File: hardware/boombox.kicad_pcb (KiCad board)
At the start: 2 copper layers, 13 parts, among them J1 Micro_SD_Card_Det1, J5 AudioJack4, U7 MCP7940MT-I/SN, U9 MCP73811T-420I-OT

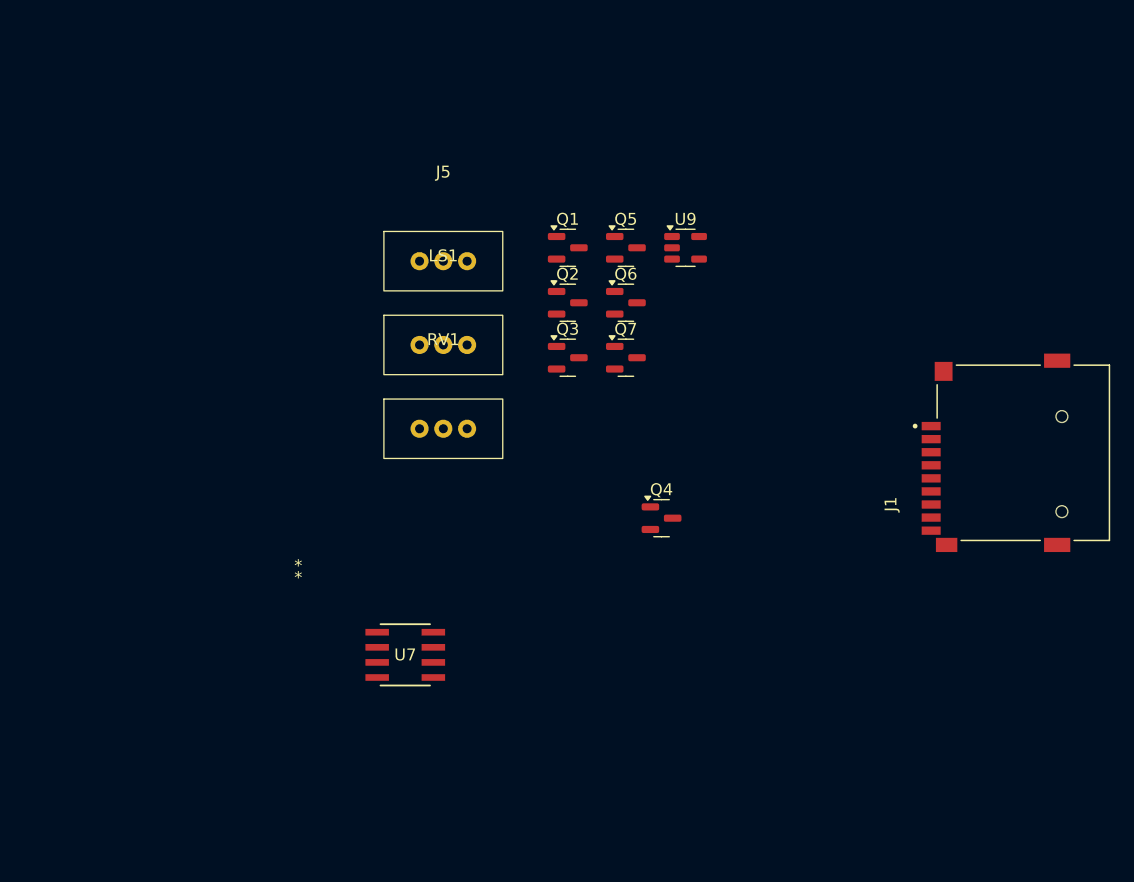
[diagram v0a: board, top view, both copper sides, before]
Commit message: Comitting so Nate can see errors
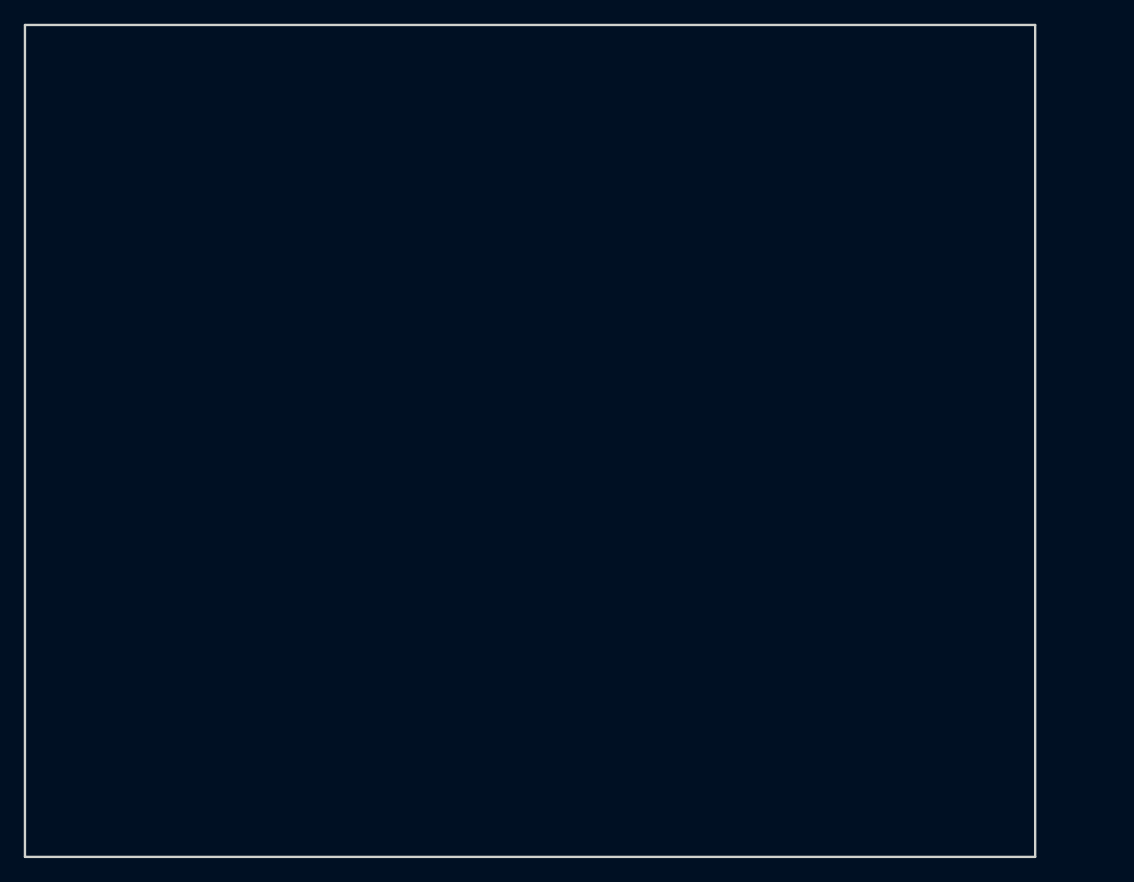
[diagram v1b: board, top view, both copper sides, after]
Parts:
- removed J1: Micro_SD_Card_Det1, boombox:CUI_MSD-4-A
- removed J5: AudioJack4, boombox:Degson 3 Pin
- removed LS1: Speaker, boombox:Degson 3 Pin
- removed Q1, Q2, Q3, Q4, Q5, Q6, Q7: ~, Package_TO_SOT_SMD:SOT-23
- removed RV1: R_Potentiometer_US, boombox:Degson 3 Pin
- removed U7: MCP7940MT-I/SN, boombox:SOIC8-N_MC_MCH
- removed U9: MCP73811T-420I-OT, Package_TO_SOT_SMD:SOT-23-5
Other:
- board outline added: 85 x 70 mm
